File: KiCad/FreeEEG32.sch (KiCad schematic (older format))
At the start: 38 parts, among them P11 CONN_01X03, SW1 NRST, SW2 SWITCH_INV, U1 ADP7118AUJZ-3.3_TSOT, U12 MPU-6500, U2 ADP7118AUJZ-3.3_TSOT, U3 8.192MHz, U37 STM32F427ZI_4side_short, U39 ADP7118AUJZ-3.3_TSOT, U43 473521001, Y2 8MHz

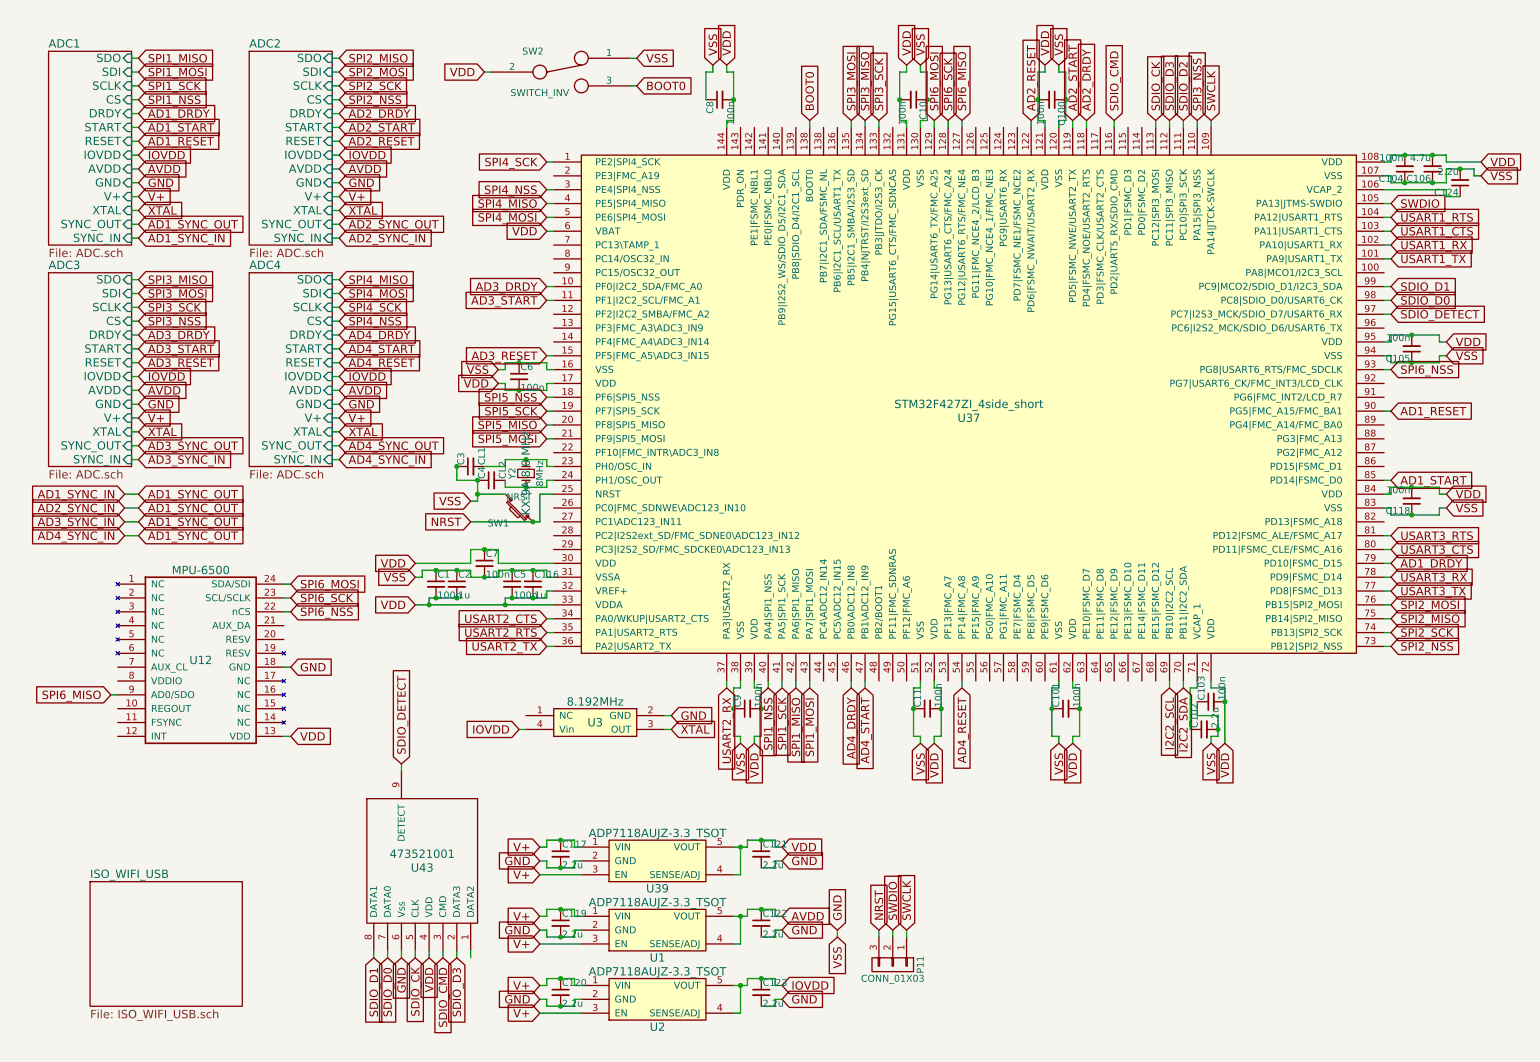
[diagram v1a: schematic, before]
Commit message: kicad
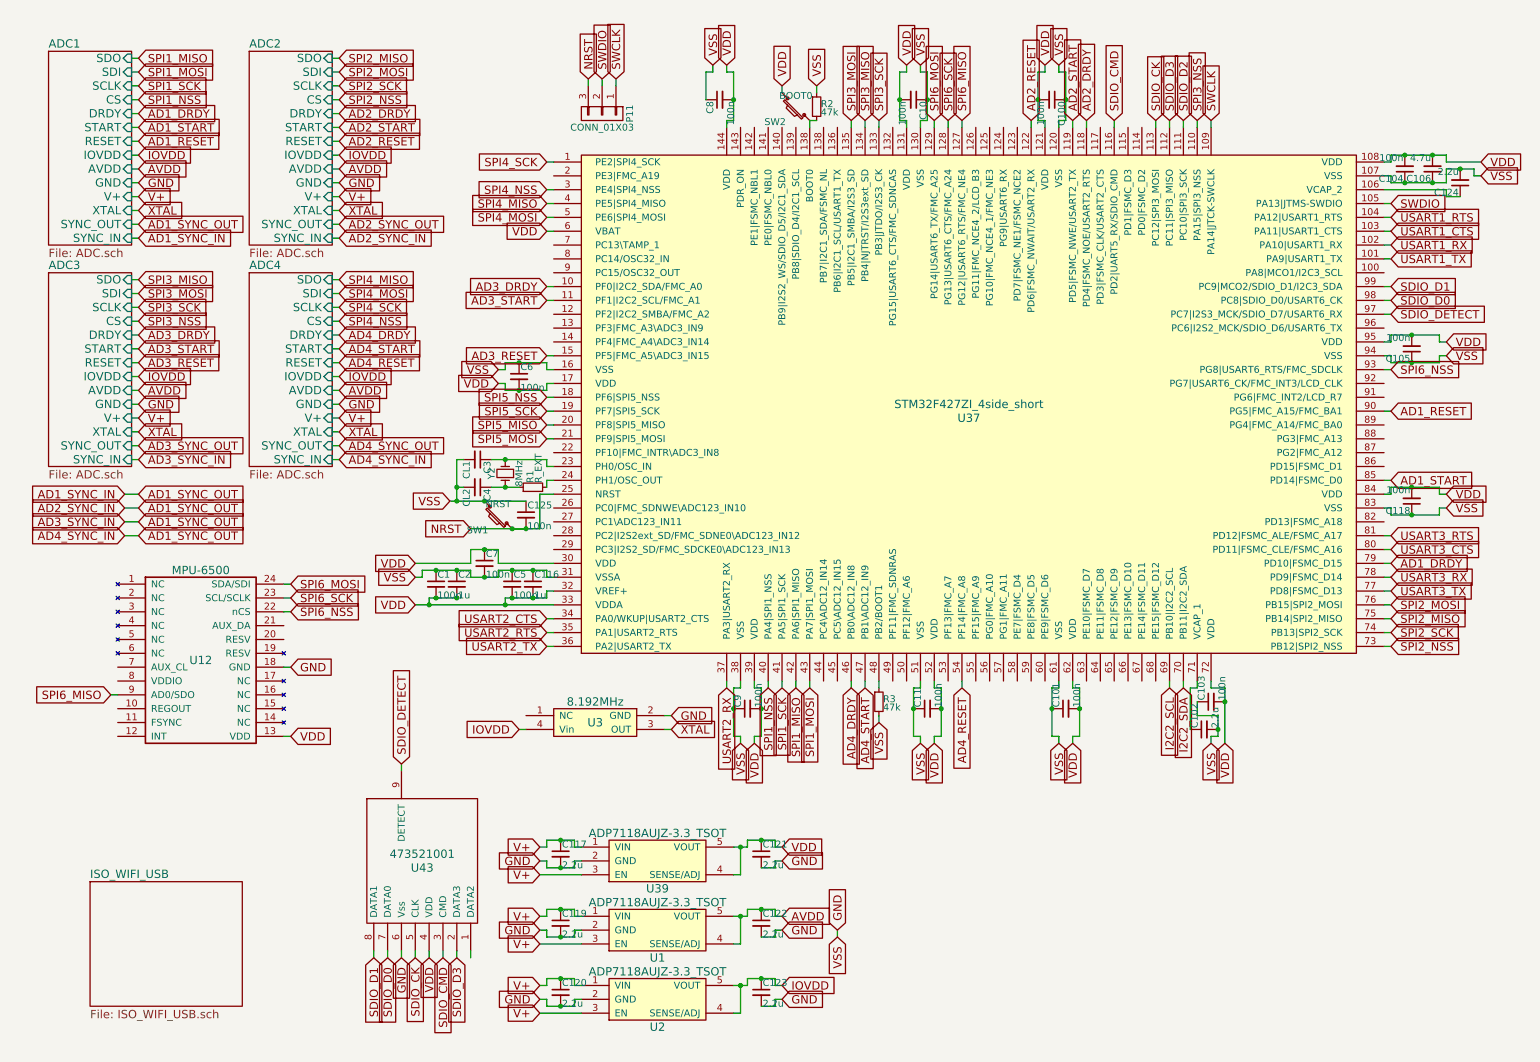
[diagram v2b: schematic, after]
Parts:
- removed SW2: SWITCH_INV, Buttons_Switches_SMD:SW_SPST_B3U-1100P-B, symbol SWITCH_INV
- added C125: 100n, Capacitors_SMD:C_0402, symbol C_Small
- added R1: R_EXT, Resistors_SMD:R_0402, symbol R_Small
- added R2, R3: 47k, Resistors_SMD:R_0402, symbol R_Small
- added SW2: BOOT0, Buttons_Switches_SMD:SW_SPST_B3U-1000P, symbol SW_PUSH_SMALL
- SW1: footprint Buttons_Switches_SMD:SW_SPST_B3U-1000P-B -> Buttons_Switches_SMD:SW_SPST_B3U-3000P-B; manf# (none) -> B3U3000PMB
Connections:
- net BOOT0 is gone; now on an unnamed net: U37.138 (PB7|I2C1_SDA/FSMC_NL)
- net GND: now also C3.2, C4.2, C125.1, R2.1, R3.2; no longer C3.1, C4.1
- net NRST: now also C125.2
- net VDD: now also SW2.2
- net at U37.23 (PH0/OSC_IN), Y2.2: now also C3.1; no longer C3.2
- net at U37.138 (PB7|I2C1_SDA/FSMC_NL): now also R2.2, SW2.1
- net at U37.48 (PB2/BOOT1): now also R3.1
- new net: C4.1, R1.1, Y2.1
- new net: R1.2, U37.24 (PH1/OSC_OUT)
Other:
- moved on the sheet: C3, C4, P11, SW1, Y2
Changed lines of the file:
@@
 L Crystal_Small Y2
 U 1 1 5841A270
-P 4050 3700
-F 0 "Y2" H 4050 3800 50  0000 C CNN
-F 1 "8MHz" H 4050 3600 50  0000 C CNN
-F 2 "Crystals:Crystal_SMD_5032_4Pads" H 4050 3700 50  0001 C CNN
-F 3 "" H 4050 3700 50  0000 C CNN
-F 4 "KX-9A 8.0 MHz" H 4050 3700 60  0000 C CNN "manf#"
-	1    4050 3700
+P 3900 3700
+F 0 "Y2" H 3900 3800 50  0000 C CNN
+F 1 "8MHz" H 3900 3600 50  0000 C CNN
+F 2 "Crystals:Crystal_SMD_5032_4Pads" H 3900 3700 50  0001 C CNN
+F 3 "" H 3900 3700 50  0000 C CNN
+F 4 "KX-9A 8.0 MHz" H 3900 3700 60  0001 C CNN "manf#"
+	1    3900 3700
 	0    -1   -1   0
 $EndComp
@@
 L C_Small C3
 U 1 1 5841A27C
-P 3650 3650
-F 0 "C3" H 3660 3720 50  0000 L CNN
-F 1 "CL1" H 3660 3570 50  0000 L CNN
-F 2 "Capacitors_SMD:C_0402" H 3650 3650 50  0001 C CNN
-F 3 "" H 3650 3650 50  0000 C CNN
-	1    3650 3650
-	0    -1   -1   0
+P 3700 3600
+F 0 "C3" H 3710 3670 50  0000 L CNN
+F 1 "CL1" H 3710 3520 50  0000 L CNN
+F 2 "Capacitors_SMD:C_0402" H 3700 3600 50  0001 C CNN
+F 3 "" H 3700 3600 50  0000 C CNN
+	1    3700 3600
+	0    1    1    0
 $EndComp
 $Comp
 L C_Small C4
 U 1 1 5841A28E
-P 3800 3750
-F 0 "C4" H 3810 3820 50  0000 L CNN
-F 1 "CL2" H 3810 3670 50  0000 L CNN
-F 2 "Capacitors_SMD:C_0402" H 3800 3750 50  0001 C CNN
-F 3 "" H 3800 3750 50  0000 C CNN
-	1    3800 3750
-	0    -1   -1   0
-$EndComp
-Text GLabel 3650 3900 0    60   Input ~ 0
+P 3700 3800
+F 0 "C4" H 3710 3870 50  0000 L CNN
+F 1 "CL2" H 3710 3720 50  0000 L CNN
+F 2 "Capacitors_SMD:C_0402" H 3700 3800 50  0001 C CNN
+F 3 "" H 3700 3800 50  0000 C CNN
+	1    3700 3800
+	0    1    1    0
+$EndComp
+Text GLabel 3500 3900 0    60   Input ~ 0
 VSS
 $Comp
@@
 L SW_PUSH_SMALL SW1
 U 1 1 5841A2AD
-P 4000 3950
-F 0 "SW1" H 4150 4060 50  0000 C CNN
-F 1 "NRST" H 4000 3871 50  0000 C CNN
-F 2 "Buttons_Switches_SMD:SW_SPST_B3U-1000P-B" H 4000 3950 50  0001 C CNN
-F 3 "" H 4000 3950 50  0000 C CNN
-	1    4000 3950
+P 3850 4000
+F 0 "SW1" H 4000 4110 50  0000 C CNN
+F 1 "NRST" H 3850 3921 50  0000 C CNN
+F 2 "Buttons_Switches_SMD:SW_SPST_B3U-3000P-B" H 3850 4000 50  0001 C CNN
+F 3 "" H 3850 4000 50  0000 C CNN
+F 4 "B3U3000PMB" H 3850 4000 60  0001 C CNN "manf#"
+	1    3850 4000
 	-1   0    0    1
 $EndComp
-Text GLabel 3650 4050 0    60   Input ~ 0
+Text GLabel 3650 4100 0    60   Input ~ 0
 NRST
 Text GLabel 10300 1750 2    60   Input ~ 0
@@
 Text GLabel 6600 1150 1    60   Input ~ 0
 SPI3_SCK
-Text GLabel 6100 1150 1    60   Input ~ 0
-BOOT0
 Text GLabel 4200 1450 0    60   Input ~ 0
 SPI4_SCK
@@
 L CONN_01X03 P11
 U 1 1 58BA2E74
-P 6700 7250
-F 0 "P11" H 6700 7450 50  0000 C CNN
-F 1 "CONN_01X03" V 6800 7250 50  0000 C CNN
-F 2 "Socket_Strips:Socket_Strip_Straight_1x03" H 6700 7250 50  0001 C CNN
-F 3 "" H 6700 7250 50  0000 C CNN
-F 4 "PBS-3" H 6700 7250 60  0001 C CNN "manf#"
-	1    6700 7250
+P 4600 1100
+F 0 "P11" H 4600 1300 50  0000 C CNN
+F 1 "CONN_01X03" V 4700 1100 50  0000 C CNN
+F 2 "Socket_Strips:Socket_Strip_Straight_1x03" H 4600 1100 50  0001 C CNN
+F 3 "" H 4600 1100 50  0000 C CNN
+F 4 "PBS-3" H 4600 1100 60  0001 C CNN "manf#"
+	1    4600 1100
 	0    1    1    0
 $EndComp
-Text GLabel 6800 7000 1    60   Input ~ 0
+Text GLabel 4700 850  1    60   Input ~ 0
 SWCLK
-Text GLabel 6700 7000 1    60   Input ~ 0
+Text GLabel 4600 850  1    60   Input ~ 0
 SWDIO
-Text GLabel 6600 7000 1    60   Input ~ 0
+Text GLabel 4500 850  1    60   Input ~ 0
 NRST
 Text GLabel 4200 4850 0    60   Input ~ 0
@@
 	4200 4950 4250 4950
 Wire Wire Line
-	3900 3800 4200 3800
+	3800 3800 4000 3800
 Wire Wire Line
 	4200 3800 4200 3750
-Connection ~ 4050 3600
-Connection ~ 4050 3800
-Wire Wire Line
-	3550 3750 3700 3750
-Wire Wire Line
-	3700 3750 3700 3900
-Connection ~ 3550 3650
-Connection ~ 3700 3750
-Wire Wire Line
-	3900 3600 4200 3600
+Connection ~ 3900 3600
+Connection ~ 3900 3800
+Wire Wire Line
+	3800 3600 4200 3600
 Connection ~ 4000 3100
 Connection ~ 4000 2900
@@
 Wire Wire Line
 	3850 2950 3900 2950
-Connection ~ 4100 4050
-Wire Wire Line
-	3700 3850 3900 3850
-Connection ~ 3700 3850
-Wire Wire Line
-	3700 3900 3650 3900
+Connection ~ 3950 4100
+Wire Wire Line
+	3500 3900 4050 3900
 Wire Wire Line
 	10250 1750 10300 1750
@@
 	6400 1200 6400 1150
 Wire Wire Line
-	6100 1150 6100 1200
-Wire Wire Line
 	4250 1850 4200 1850
 Wire Wire Line
@@
 	10250 1850 10300 1850
 Wire Wire Line
-	6800 7000 6800 7050
-Wire Wire Line
-	6700 7000 6700 7050
-Wire Wire Line
-	6600 7000 6600 7050
+	4700 850  4700 900
+Wire Wire Line
+	4600 850  4600 900
+Wire Wire Line
+	4500 850  4500 900
 Wire Wire Line
 	4250 4750 4200 4750
@@
 Wire Wire Line
 	4200 3600 4200 3650
-Wire Wire Line
-	3900 3600 3900 3650
-Wire Wire Line
-	3900 3650 3750 3650
-Wire Wire Line
-	3550 3750 3550 3650
-Wire Wire Line
-	3900 3800 3900 3750
 Wire Wire Line
 	5600 6400 5600 6600
@@
 Wire Wire Line
 	4200 1950 4250 1950
-Text GLabel 4850 700  2    60   Input ~ 0
-VSS
-Text GLabel 3750 800  0    60   Input ~ 0
-VDD
-Wire Wire Line
-	3800 800  3750 800
-Wire Wire Line
-	4800 700  4850 700
-Text GLabel 4850 900  2    60   Input ~ 0
-BOOT0
-$Comp
-L SWITCH_INV SW2
-U 1 1 58E042BC
-P 4300 800
-F 0 "SW2" H 4100 950 50  0000 C CNN
-F 1 "SWITCH_INV" H 4150 650 50  0000 C CNN
-F 2 "Buttons_Switches_SMD:SW_SPST_B3U-1100P-B" H 4300 800 50  0001 C CNN
-F 3 "" H 4300 800 50  0000 C CNN
-	1    4300 800
-	1    0    0    -1
-$EndComp
-Wire Wire Line
-	4850 900  4800 900
-Wire Wire Line
-	4150 4050 4150 3850
+Wire Wire Line
+	4150 4100 4150 3850
 Wire Wire Line
 	4150 3850 4250 3850
 Wire Wire Line
-	4150 4050 3650 4050
+	3650 4100 4150 4100
 $Comp
 L MPU-6500 U12
@@
 	1    0    0    -1
 $EndComp
+Text GLabel 6600 5500 3    60   Input ~ 0
+VSS
+Wire Wire Line
+	6600 5200 6600 5250
+$Comp
+L C_Small C125
+U 1 1 58E42B84
+P 4050 4000
+F 0 "C125" H 4060 4070 50  0000 L CNN
+F 1 "100n" H 4060 3920 50  0000 L CNN
+F 2 "Capacitors_SMD:C_0402" H 4050 4000 50  0001 C CNN
+F 3 "" H 4050 4000 50  0000 C CNN
+F 4 "MC0402B104K160CT" H 4050 4000 60  0001 C CNN "manf#"
+	1    4050 4000
+	1    0    0    -1
+$EndComp
+Wire Wire Line
+	3950 4100 4050 4100
+Connection ~ 4050 4100
+Connection ~ 3750 3900
+$Comp
+L R_Small R1
+U 1 1 58E45491
+P 4100 3800
+F 0 "R1" H 4130 3820 50  0000 L CNN
+F 1 "R_EXT" H 4130 3760 50  0000 L CNN
+F 2 "Resistors_SMD:R_0402" H 4100 3800 50  0001 C CNN
+F 3 "" H 4100 3800 50  0000 C CNN
+	1    4100 3800
+	0    -1   -1   0
+$EndComp
+Wire Wire Line
+	3600 3600 3550 3600
+Wire Wire Line
+	3550 3600 3550 3900
+Wire Wire Line
+	3600 3800 3550 3800
+Connection ~ 3550 3800
+Connection ~ 3550 3900
+$Comp
+L R_Small R3
+U 1 1 58E49D48
+P 6600 5350
+F 0 "R3" H 6630 5370 50  0000 L CNN
+F 1 "47k" H 6630 5310 50  0000 L CNN
+F 2 "Resistors_SMD:R_0402" H 6600 5350 50  0001 C CNN
+F 3 "" H 6600 5350 50  0000 C CNN
+F 4 "RC0402FR-0747KL" H 6600 5350 60  0001 C CNN "manf#"
+	1    6600 5350
+	1    0    0    -1
+$EndComp
+Wire Wire Line
+	6600 5500 6600 5450
+$Comp
+L R_Small R2
+U 1 1 58E4B6DE
+P 6150 1050
+F 0 "R2" H 6180 1070 50  0000 L CNN
+F 1 "47k" H 6180 1010 50  0000 L CNN
+F 2 "Resistors_SMD:R_0402" H 6150 1050 50  0001 C CNN
+F 3 "" H 6150 1050 50  0000 C CNN
+F 4 "RC0402FR-0747KL" H 6150 1050 60  0001 C CNN "manf#"
+	1    6150 1050
+	1    0    0    -1
+$EndComp
+Text GLabel 6150 900  1    60   Input ~ 0
+VSS
+Wire Wire Line
+	6150 950  6150 900
+$Comp
+L SW_PUSH_SMALL SW2
+U 1 1 58E4FE38
+P 6000 1050
+F 0 "SW2" H 6150 1160 50  0000 C CNN
+F 1 "BOOT0" H 6000 971 50  0000 C CNN
+F 2 "Buttons_Switches_SMD:SW_SPST_B3U-1000P" H 6000 1050 50  0001 C CNN
+F 3 "" H 6000 1050 50  0000 C CNN
+F 4 "B3U1000P" H 6000 1050 60  0001 C CNN "manf#"
+	1    6000 1050
+	-1   0    0    1
+$EndComp
+Text GLabel 5900 900  1    60   Input ~ 0
+VDD
+Wire Wire Line
+	6100 1200 6100 1150
+Wire Wire Line
+	6100 1150 6150 1150
+Wire Wire Line
+	5900 950  5900 900
 $EndSCHEMATC
